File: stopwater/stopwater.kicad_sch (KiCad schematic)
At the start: 56 parts, among them J1 USB_B_Micro, J10 Conn_01x06_Socket, J18 Out, J19 Out, J2 ~220, J3 Conn_01x06_Pin, J4 Conn_01x02_Pin, J5 Out, J6 Conn_01x02_Socket, J7 Conn_01x02_Pin, J8 Conn_01x02_Socket, J9 Conn_01x02_Pin, K1 G5LE-1, Q1 BC847, U1 TNY268P, U2 LD1117S33TR_SOT223, U4 TLP181

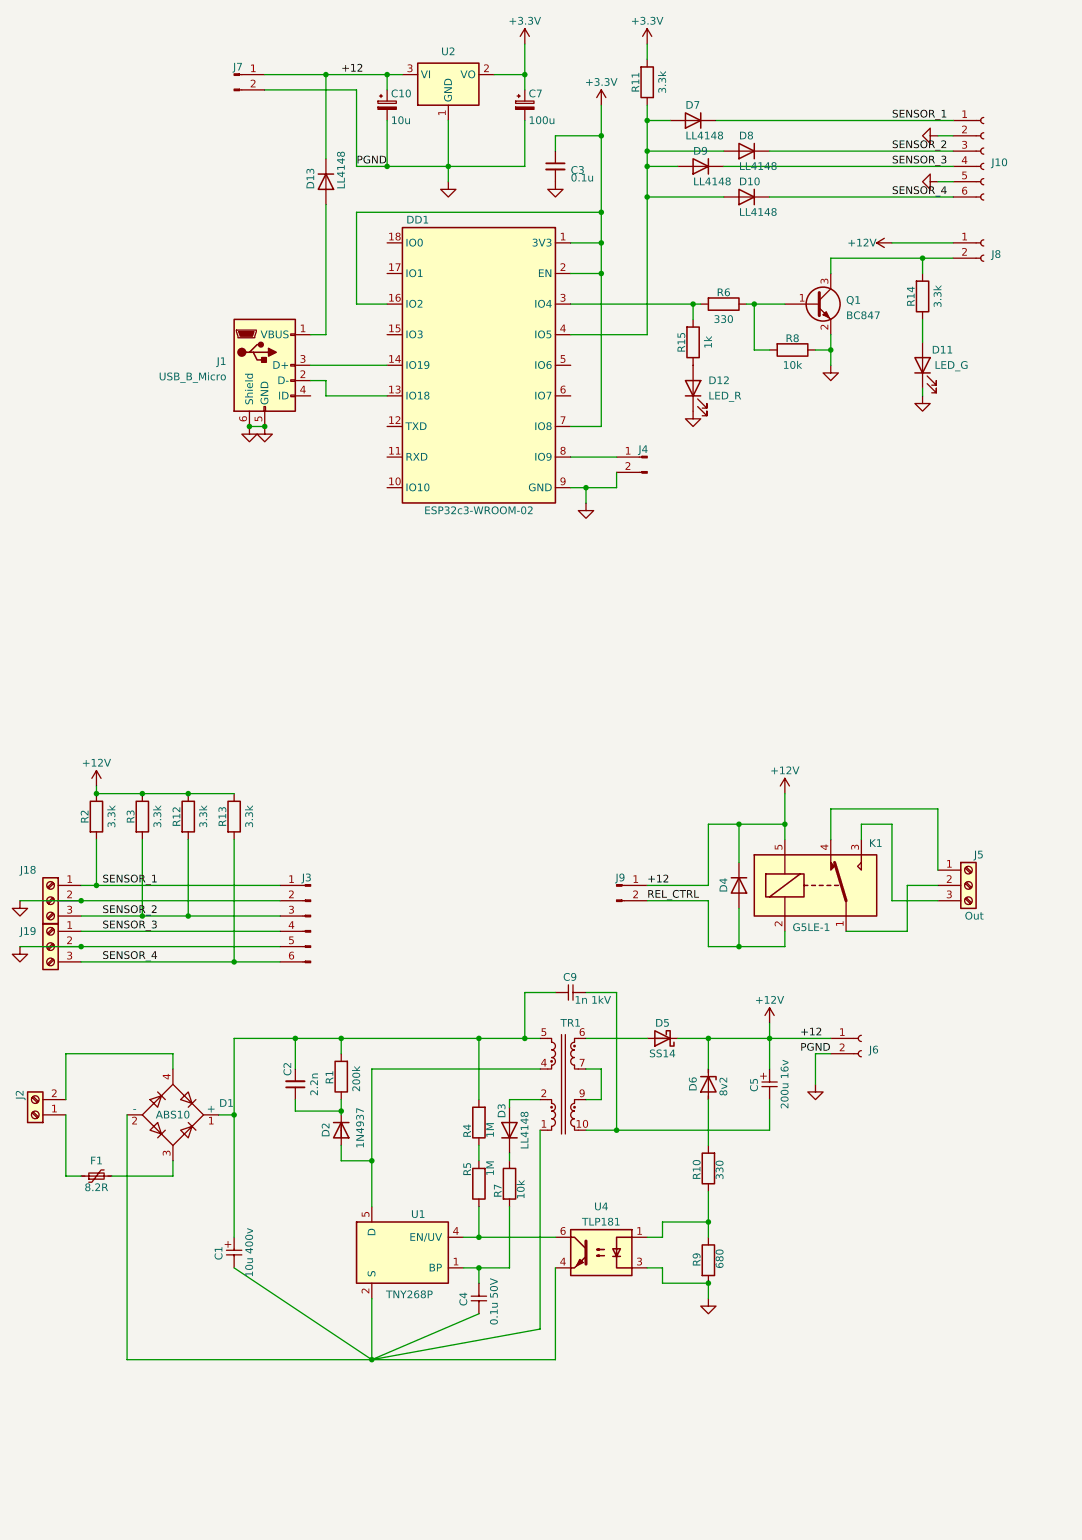
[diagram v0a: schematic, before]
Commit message: added some schematics
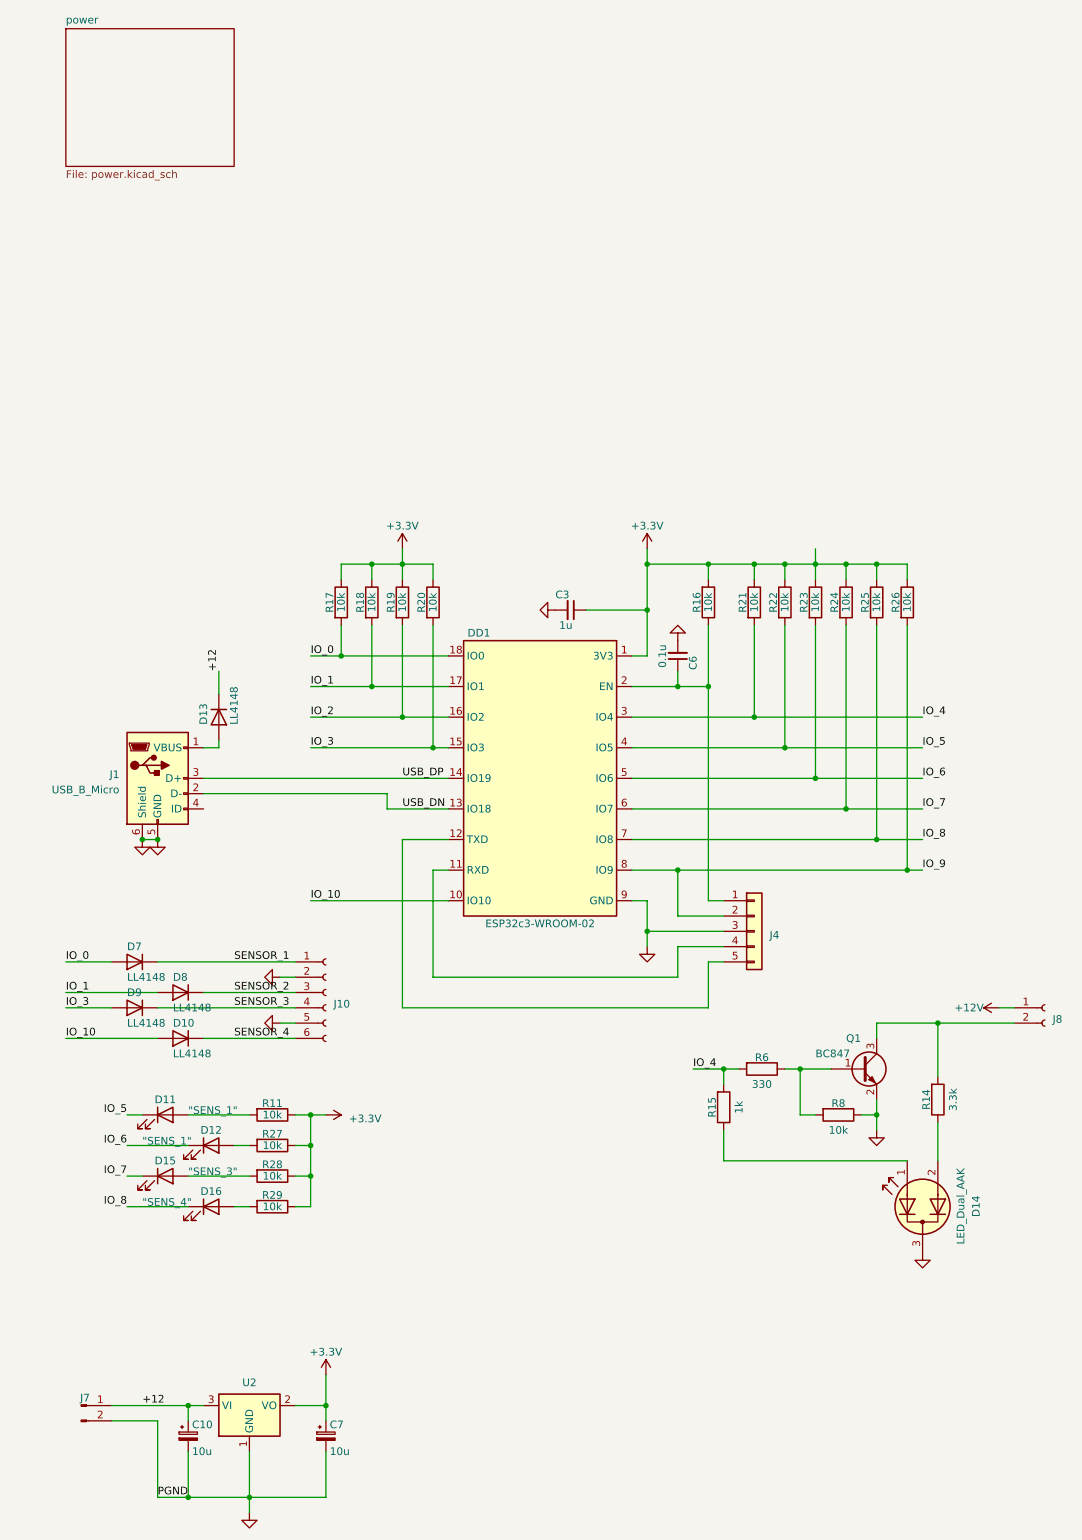
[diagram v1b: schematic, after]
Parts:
- removed C1: 10u 400v, Capacitor_THT:CP_Radial_D10.0mm_P5.00mm, symbol stopwater:C_Polarized_Small
- removed C2: 2.2n, Capacitor_THT:C_Axial_L5.1mm_D3.1mm_P7.50mm_Horizontal, symbol Device:C_Small
- removed C4: C_Polarized_Small, Capacitor_SMD:C_0805_2012Metric_Pad1.18x1.45mm_HandSolder, symbol stopwater:C
- removed C5: 200u 16v, Capacitor_THT:CP_Radial_D8.0mm_P3.50mm, symbol stopwater:C_Polarized_Small
- removed C9: C_Polarized_Small, Capacitor_THT:C_Disc_D4.3mm_W1.9mm_P5.00mm, symbol stopwater:C
- removed D1: ABS10, Diode_SMD:Diode_Bridge_Diotec_ABS, symbol Diode_Bridge:ABS10
- removed D2: 1N4937, Diode_THT:D_DO-41_SOD81_P10.16mm_Horizontal, symbol stopwater:1N4937
- removed D3: LL4148, Diode_SMD:D_MiniMELF, symbol Diode:LL4148
- removed D4: MMSD4148, Diode_SMD:D_SOD-123, symbol Diode:MMSD4148
- removed D5: SS14, Diode_SMD:D_SMA, symbol stopwater:1N5819
- removed D6: 8v2, Diode_SMD:D_MiniMELF_Handsoldering, symbol Device:D_Zener
- removed F1: 8.2R, Fuse:Fuse_BelFuse_0ZRE0005FF_L8.3mm_W3.8mm, symbol Device:Polyfuse_Small
- removed J18, J19, J5: Out, TerminalBlock_MetzConnect:TerminalBlock_MetzConnect_Type011_RT05503HBWC_1x03_P5.00mm_Horizontal, symbol Connector:Screw_Terminal_01x03
- removed J2: ~220, TerminalBlock_MetzConnect:TerminalBlock_MetzConnect_Type011_RT05502HBWC_1x02_P5.00mm_Horizontal, symbol Connector:Screw_Terminal_01x02
- removed J3: Conn_01x06_Pin, Connector_PinHeader_2.54mm:PinHeader_1x06_P2.54mm_Vertical, symbol Connector:Conn_01x06_Pin
- removed J4: Conn_01x02_Pin, Connector_PinSocket_2.54mm:PinSocket_1x02_P2.54mm_Vertical, symbol Connector:Conn_01x02_Pin
- removed J6: Conn_01x02_Socket, symbol Connector:Conn_01x02_Socket
- removed J9: Conn_01x02_Pin, symbol Connector:Conn_01x02_Pin
- removed K1: G5LE-1, Relay_THT:Relay_SPDT_Omron-G5LE-1, symbol Relay:G5LE-1
- removed R1: 200k, Resistor_THT:R_Axial_DIN0411_L9.9mm_D3.6mm_P15.24mm_Horizontal, symbol Device:R
- removed R10: 330, Resistor_SMD:R_0805_2012Metric_Pad1.20x1.40mm_HandSolder, symbol Device:R
- removed R12, R13, R2, R3: 3.3k, Resistor_SMD:R_0603_1608Metric_Pad0.98x0.95mm_HandSolder, symbol Device:R
- removed R4, R5: 1M, Resistor_SMD:R_1206_3216Metric_Pad1.30x1.75mm_HandSolder, symbol Device:R
- removed R7: 10k, Resistor_SMD:R_0805_2012Metric_Pad1.20x1.40mm_HandSolder, symbol Device:R
- removed R9: 680, Resistor_SMD:R_0805_2012Metric_Pad1.20x1.40mm_HandSolder, symbol Device:R
- removed TR1: FAT_74082, stopwater:FAT_74082, symbol stopwater:FAT_74082
- removed U1: TNY268P, Package_DIP:PowerIntegrations_PDIP-8B, symbol Regulator_Switching:TNY268P
- removed U4: TLP181, Package_SO:SOIC-4_4.55x3.7mm_P2.54mm, symbol Isolator:TLP185
- added C6: 0.1u, Capacitor_SMD:C_0603_1608Metric_Pad1.08x0.95mm_HandSolder, symbol Device:C_Small
- added D14: LED_Dual_AAK, LED_SMD:LED_Cree-XB, symbol Device:LED_Dual_AAK
- added D15: "SENS_3", LED_SMD:LED_0805_2012Metric, symbol Device:LED
- added D16: "SENS_4", LED_SMD:LED_0805_2012Metric, symbol Device:LED
- added J4: Conn_01x05, Connector_PinHeader_2.54mm:PinHeader_1x05_P2.54mm_Vertical, symbol Connector_Generic:Conn_01x05
- added R16, R17, R18, R19, R20, R21, R22, R23, R24, R25, R26, R27, R28, R29: 10k, Resistor_SMD:R_0603_1608Metric, symbol Device:R
- C10: footprint Capacitor_THT:CP_Radial_D5.0mm_P2.50mm -> Capacitor_Tantalum_SMD:CP_EIA-3528-15_AVX-H
- C3: value 0.1u -> 1u; footprint Capacitor_SMD:C_0603_1608Metric_Pad1.08x0.95mm_HandSolder -> Capacitor_SMD:C_0805_2012Metric
- C7: value 100u -> 10u; footprint Capacitor_Tantalum_SMD:CP_EIA-2012-12_Kemet-R -> Capacitor_Tantalum_SMD:CP_EIA-3528-15_AVX-H
- D11: value LED_G -> "SENS_1"; footprint (none) -> LED_SMD:LED_0805_2012Metric
- D12: value LED_R -> "SENS_1"; footprint (none) -> LED_SMD:LED_0805_2012Metric
- DD1: footprint stopwater:ESP32C3-WROOM-02 -> stopwater:ESP-WROOM-02
- J10: footprint (none) -> Connector_PinHeader_2.54mm:PinHeader_1x06_P2.54mm_Vertical
- J7, J8: footprint (none) -> Connector_PinHeader_2.54mm:PinHeader_1x02_P2.54mm_Vertical
- R11: value 3.3k -> 10k; footprint Resistor_SMD:R_0603_1608Metric_Pad0.98x0.95mm_HandSolder -> Resistor_SMD:R_0603_1608Metric
- R14, R15, R6, R8: footprint Resistor_SMD:R_0603_1608Metric_Pad0.98x0.95mm_HandSolder -> Resistor_SMD:R_0603_1608Metric
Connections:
- net +12V: no longer C10.1, D13.1 (K), J7.1 (Pin_1), U2.3 (VI)
- net +3.3V: now also R11.1, R16.2, R17.1, R18.1, R19.1, R20.1, R21.1, R22.1, R23.1, R24.1, R25.1, R26.1, R27.1, R28.1, R29.1; no longer DD1.16 (IO2), DD1.2 (EN), DD1.7 (IO8), R11.2
- net GND: now also C6.2, D14.3 (K), J4.3 (Pin_3); no longer D11.1 (K), D12.1 (K)
- net at D11.2 (A): now also R11.2; no longer R14.1
- net IO_4: now reaches DD1.3 (IO4), R15.2, R6.2
- net IO_4: now also R21.2
- net IO_10: now reaches DD1.10 (IO10)
- net IO_10: now also D10.2 (A)
- net at DD1.11 (RXD): now also J4.4 (Pin_4)
- net at DD1.12 (TXD): now also J4.5 (Pin_5)
- net USB_DN: now reaches DD1.13 (IO18), J1.2 (D-)
- net USB_DP: now reaches DD1.14 (IO19), J1.3 (D+)
- net IO_3: now reaches DD1.15 (IO3)
- net IO_3: now also D9.2 (A), R20.2
- net IO_1: now reaches DD1.17 (IO1)
- net IO_1: now also D8.2 (A), R18.2
- net IO_0: now reaches DD1.18 (IO0)
- net IO_0: now also D7.2 (A), R17.2
- net IO_6: now reaches DD1.5 (IO6)
- net IO_6: now also D12.1 (K), R23.2
- net IO_7: now reaches DD1.6 (IO7)
- net IO_7: now also D15.1 (K), R24.2
- net IO_9: now reaches DD1.8 (IO9)
- net IO_9: now also J4.2 (Pin_2), R26.2
- net at R15.1: now also D14.1 (A1); no longer D12.2 (A)
- new net: D15.2 (A), R28.2
- new net: D14.2 (A2), R14.1
- new net: D16.2 (A), R29.2
- new net: C6.1, DD1.2 (EN), J4.1 (Pin_1), R16.1
- new net: D12.2 (A), R27.2
- new net +12: C10.1, D13.1 (K), J7.1 (Pin_1), U2.3 (VI)
- new net IO_2: DD1.16 (IO2), R19.2
- new net IO_5: D11.1 (K), DD1.4 (IO5), R22.2
- new net IO_8: D16.1 (K), DD1.7 (IO8), R25.2
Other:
- added sheet power (power.kicad_sch)
- moved on the sheet: C10, C3, C7, D10, D13, D7, D8, D9, DD1, J1, J10, J7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
